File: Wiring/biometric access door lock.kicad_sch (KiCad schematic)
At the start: 16 parts, among them U1 ESP32-WROOM-32

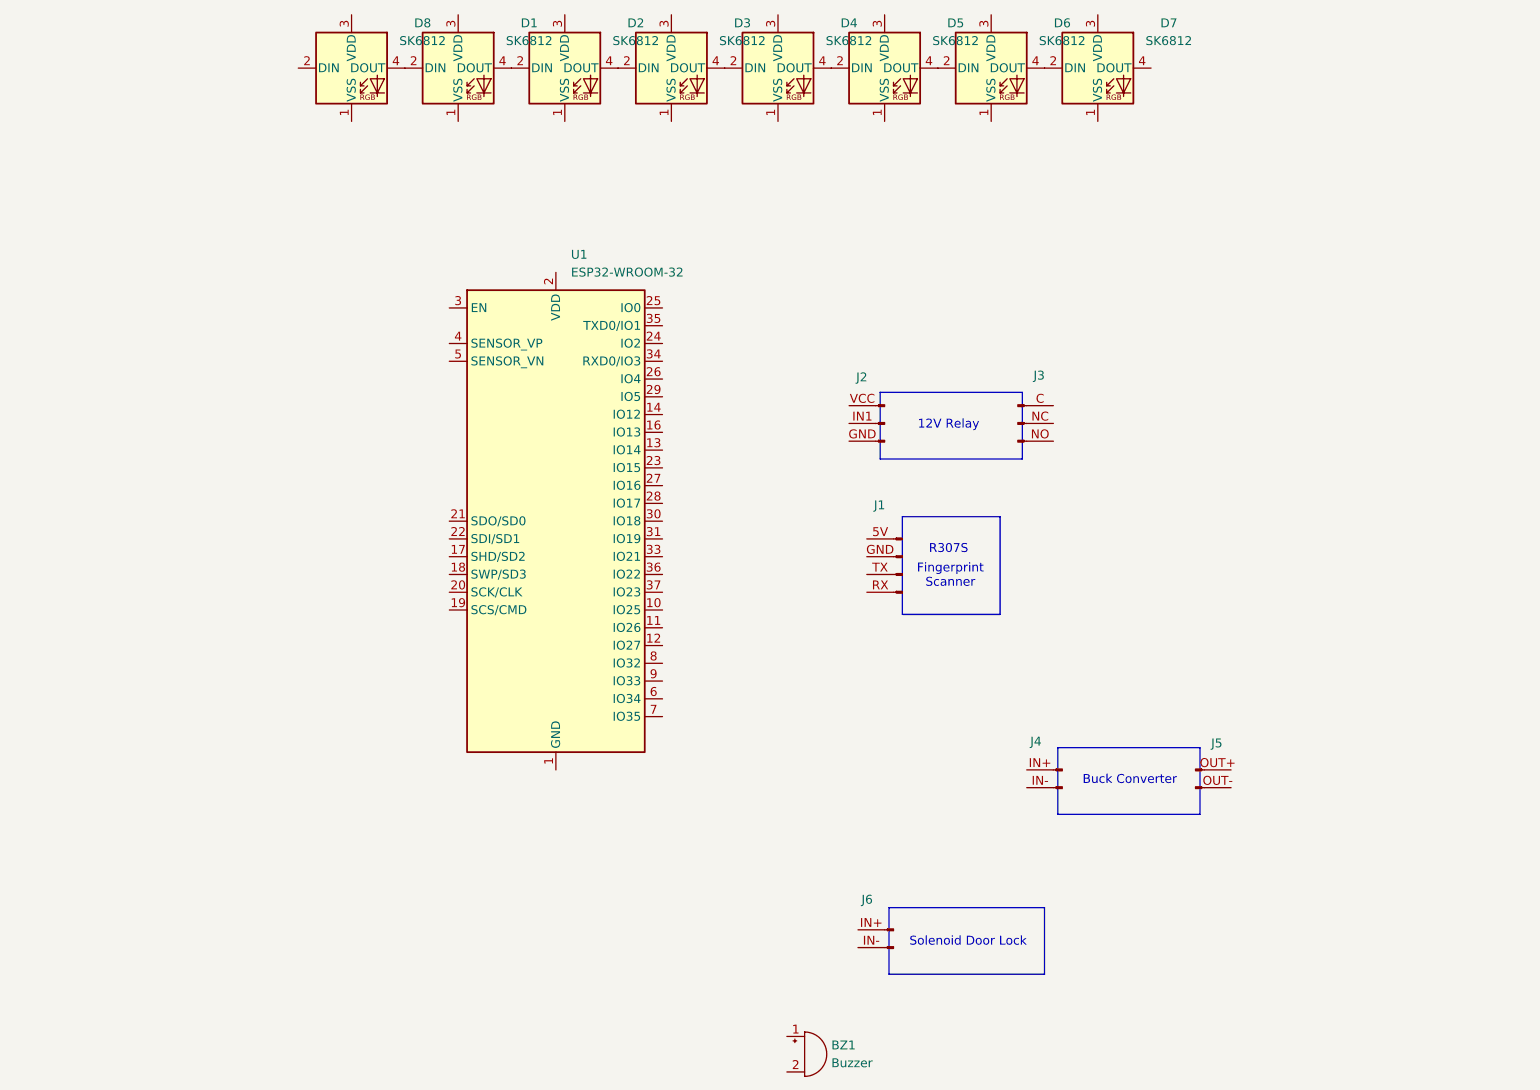
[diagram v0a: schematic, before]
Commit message: wiring complete
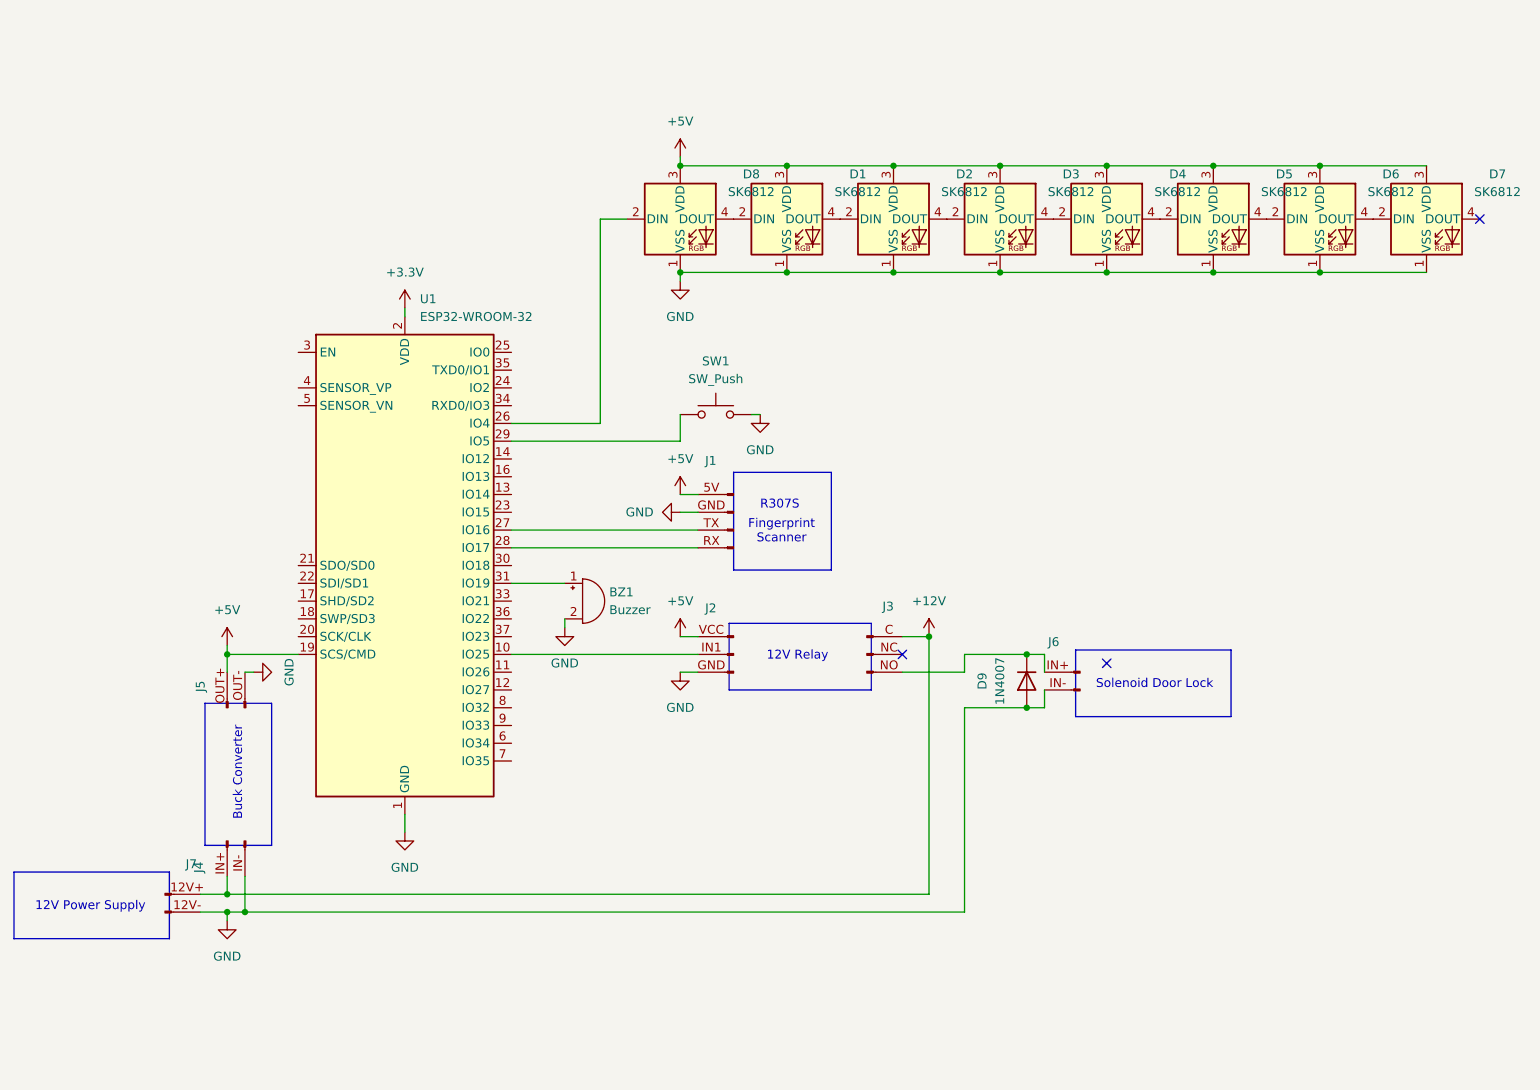
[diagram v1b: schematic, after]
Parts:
- added D9: 1N4007, Diode_THT:D_DO-41_SOD81_P10.16mm_Horizontal, symbol Diode:1N4007
- added J7: ~, symbol Connector:Conn_01x02_Pin
- added SW1: SW_Push, symbol Switch:SW_Push
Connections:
- net GND: now reaches D6.1 (VSS)
- net GND: now also BZ1.2 (-), D1.1 (VSS), D2.1 (VSS), D3.1 (VSS), D4.1 (VSS), D5.1 (VSS), D7.1 (VSS), D8.1 (VSS), J1.GND (Pin_2), J2.GND (Pin_3), J4.IN- (Pin_2), J5.OUT- (Pin_2), J6.IN- (Pin_2), U1.1 (GND), U1.15 (GND), U1.38 (GND), U1.39 (GND), D9.2 (A), J7.12V- (Pin_2), SW1.2
- net +5V: now reaches D6.3 (VDD)
- net +5V: now also D1.3 (VDD), D2.3 (VDD), D3.3 (VDD), D4.3 (VDD), D5.3 (VDD), D7.3 (VDD), D8.3 (VDD), J1.5V (Pin_1), J2.VCC (Pin_1), J5.OUT+ (Pin_1), U1.19 (SCS/CMD)
- net at D8.2 (DIN): now also U1.26 (IO4)
- net at J6.IN+ (Pin_1): now also J3.NO (Pin_3), D9.1 (K)
- net +12V: now reaches J3.C (Pin_1)
- net +12V: now also J4.IN+ (Pin_1), J7.12V+ (Pin_1)
- net at BZ1.1 (+): now also U1.31 (IO19)
- net at J2.IN1 (Pin_2): now also U1.10 (IO25)
- net at J1.RX (Pin_4): now also U1.28 (IO17)
- net at J1.TX (Pin_3): now also U1.27 (IO16)
- net +3.3V: now reaches U1.2 (VDD)
- net at U1.29 (IO5): now also SW1.1
- no-connect marks 0 -> 3
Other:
- note added: "12V Power Supply"
- moved on the sheet: BZ1, D1, D2, D3, D4, D5, D6, D7, D8, J1, J2, J3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
